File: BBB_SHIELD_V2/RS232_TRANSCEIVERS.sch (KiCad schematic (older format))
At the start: 13 parts, among them J4 Conn_02x05_Odd_Even

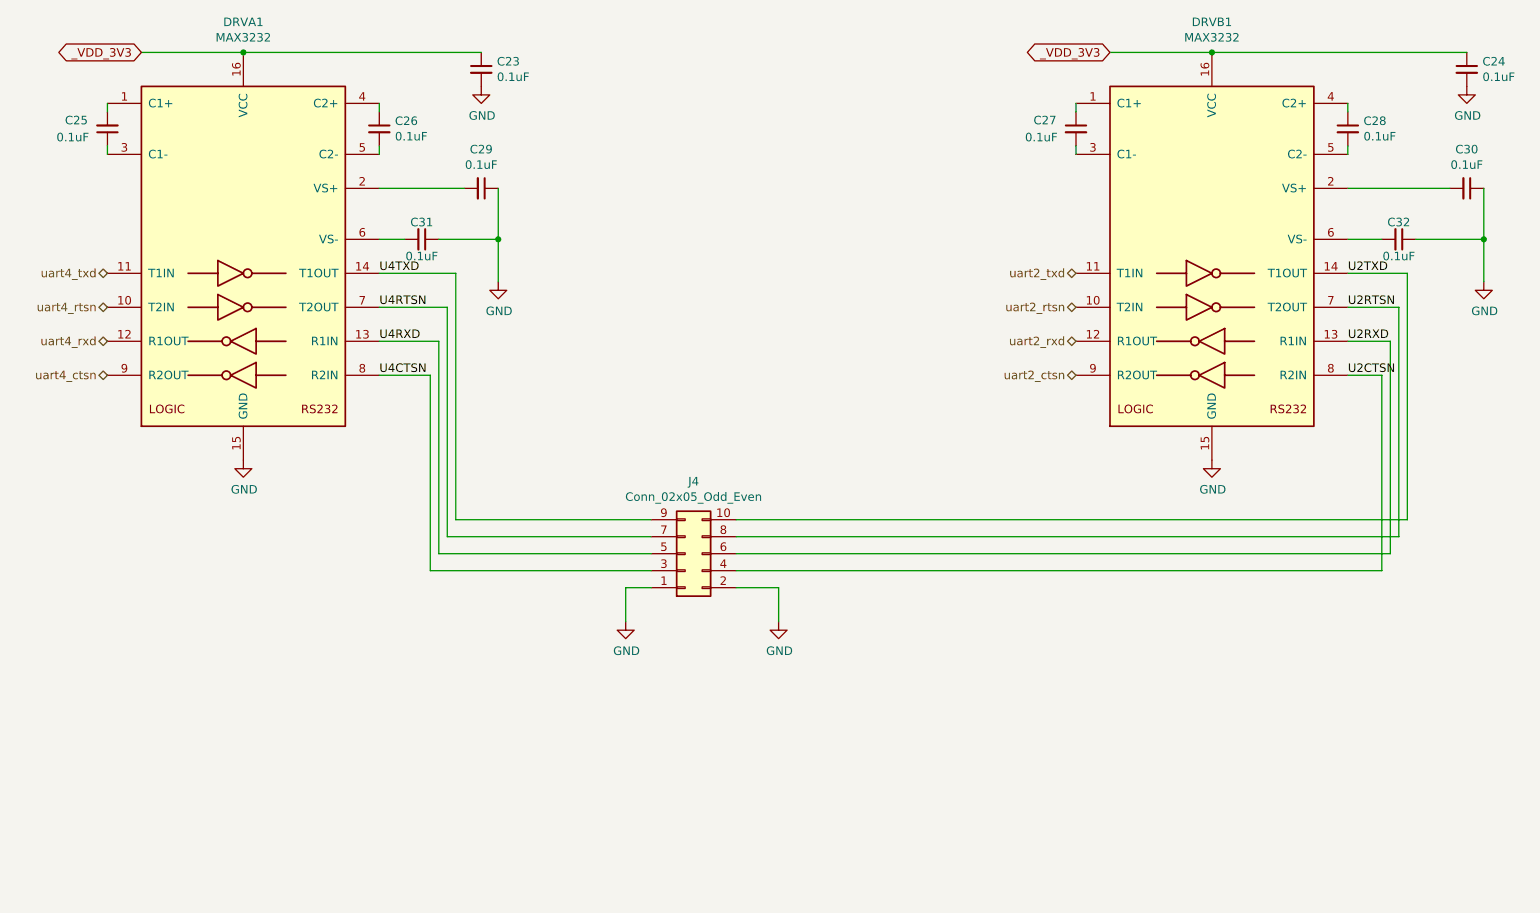
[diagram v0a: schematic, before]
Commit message: Schematic cleanup and refinement.
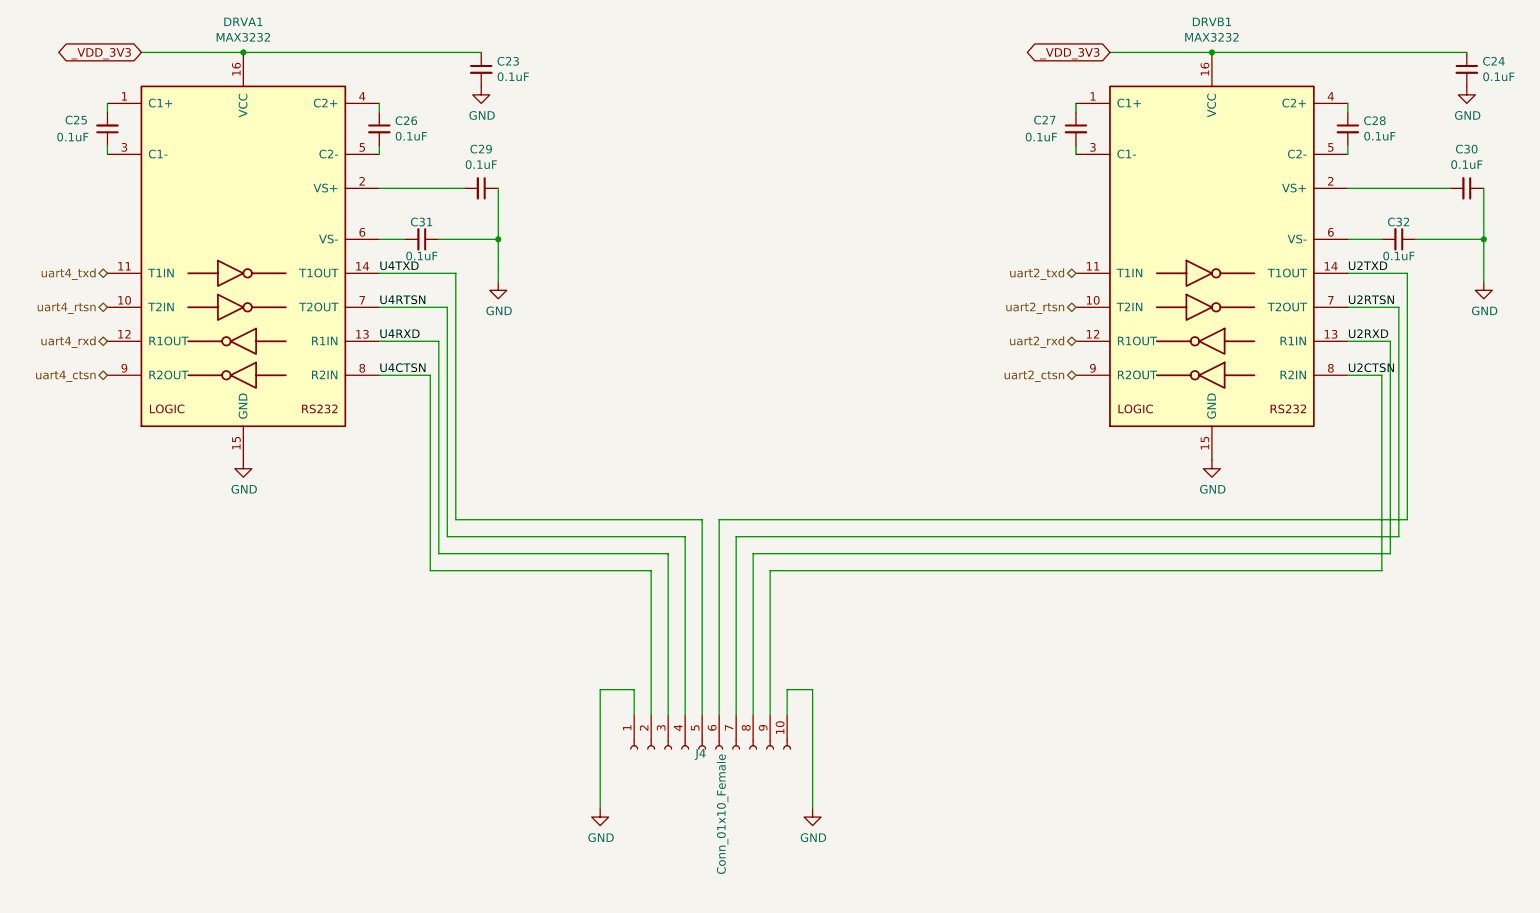
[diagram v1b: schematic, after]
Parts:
- removed J4: Conn_02x05_Odd_Even, CUSTOM_FOOTPRINTS:PCB TERMINAL BLOCK - 1841526, symbol Connector_Generic:Conn_02x05_Odd_Even
- added J4: Conn_01x10_Female, CUSTOM_FOOTPRINTS:10_POS_SPRING_TERM, symbol Connector:Conn_01x10_Female
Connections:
- net GND: now also J4.1 (Pin_1), J4.10 (Pin_10)
- net U2CTSN: now also J4.9 (Pin_9)
- net U2RTSN: now also J4.7 (Pin_7)
- net U2RXD: now also J4.8 (Pin_8)
- net U2TXD: now also J4.6 (Pin_6)
- net U4CTSN: now also J4.2 (Pin_2)
- net U4RTSN: now also J4.4 (Pin_4)
- net U4RXD: now also J4.3 (Pin_3)
- net U4TXD: now also J4.5 (Pin_5)
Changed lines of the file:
@@
 	1550 2600 2150 2600
 Connection ~ 2150 2600
-$Comp
-L Connector_Generic:Conn_02x05_Odd_Even J4
-U 1 1 5BF40240
-P 4750 5550
-F 0 "J4" H 4800 5125 50  0000 C CNN
-F 1 "Conn_02x05_Odd_Even" H 4800 5216 50  0000 C CNN
-F 2 "CUSTOM_FOOTPRINTS:PCB TERMINAL BLOCK - 1841526" H 4750 5550 50  0001 C CNN
-F 3 "" H 4750 5550 50  0001 C CNN
-F 4 "277-10318-ND" H 4750 5550 50  0001 C CNN "DKPN"
-F 5 "1841526" H 4750 5550 50  0001 C CNN "MFGPN"
-F 6 "BULK, VER 2018-12-09" H 0   0   50  0001 C CNN "NOTES"
-	1    4750 5550
-	1    0    0    1
-$EndComp
 Wire Wire Line
 	2950 3900 3400 3900
@@
 	3250 5650 4550 5650
 Wire Wire Line
-	3300 5550 4550 5550
-Wire Wire Line
-	3350 5450 4550 5450
-Wire Wire Line
-	3400 5350 4550 5350
-Wire Wire Line
 	8650 4100 8950 4100
 Wire Wire Line
@@
 	8900 4300 8900 5550
 Wire Wire Line
-	8900 5550 5050 5550
-Wire Wire Line
-	5050 5650 8850 5650
+	8900 5550 5150 5550
 Wire Wire Line
 	8850 5650 8850 4500
@@
 	8650 3900 9000 3900
 Wire Wire Line
-	5050 5350 9000 5350
-Wire Wire Line
 	9000 3900 9000 5350
-Wire Wire Line
-	4550 5750 4400 5750
-Wire Wire Line
-	4400 5750 4400 5950
-Wire Wire Line
-	5050 5750 5300 5750
-Wire Wire Line
-	5300 5750 5300 5950
 $Comp
 L power:GND #PWR054
 U 1 1 5BF49E20
-P 5300 5950
-F 0 "#PWR054" H 5300 5700 50  0001 C CNN
-F 1 "GND" H 5305 5777 50  0000 C CNN
-F 2 "" H 5300 5950 50  0001 C CNN
-F 3 "" H 5300 5950 50  0001 C CNN
-	1    5300 5950
+P 5500 7050
+F 0 "#PWR054" H 5500 6800 50  0001 C CNN
+F 1 "GND" H 5505 6877 50  0000 C CNN
+F 2 "" H 5500 7050 50  0001 C CNN
+F 3 "" H 5500 7050 50  0001 C CNN
+	1    5500 7050
 	1    0    0    -1
 $EndComp
@@
 L power:GND #PWR053
 U 1 1 5BF49E69
-P 4400 5950
-F 0 "#PWR053" H 4400 5700 50  0001 C CNN
-F 1 "GND" H 4405 5777 50  0000 C CNN
-F 2 "" H 4400 5950 50  0001 C CNN
-F 3 "" H 4400 5950 50  0001 C CNN
-	1    4400 5950
+P 4250 7050
+F 0 "#PWR053" H 4250 6800 50  0001 C CNN
+F 1 "GND" H 4255 6877 50  0000 C CNN
+F 2 "" H 4250 7050 50  0001 C CNN
+F 3 "" H 4250 7050 50  0001 C CNN
+	1    4250 7050
 	1    0    0    -1
 $EndComp
@@
 Text Label 2950 4500 0    50   ~ 0
 U4CTSN
+$Comp
+L Connector:Conn_01x10_Female J4
+U 1 1 5D15C1E2
+P 4850 6700
+F 0 "J4" V 4877 6676 50  0000 L CNN
+F 1 "Conn_01x10_Female" H 4877 6585 50  0000 L CNN
+F 2 "CUSTOM_FOOTPRINTS:10_POS_SPRING_TERM" H 4850 6700 50  0001 C CNN
+F 3 "~" H 4850 6700 50  0001 C CNN
+	1    4850 6700
+	0    -1   1    0
+$EndComp
+Wire Wire Line
+	4250 6350 4450 6350
+Wire Wire Line
+	4450 6350 4450 6500
+Wire Wire Line
+	4250 6350 4250 7050
+Wire Wire Line
+	5350 6500 5350 6350
+Wire Wire Line
+	5350 6350 5500 6350
+Wire Wire Line
+	5500 6350 5500 7050
+Wire Wire Line
+	4550 5650 4550 6500
+Wire Wire Line
+	4650 5550 4650 6500
+Wire Wire Line
+	3300 5550 4650 5550
+Wire Wire Line
+	4750 5450 4750 6500
+Wire Wire Line
+	3350 5450 4750 5450
+Wire Wire Line
+	4850 5350 4850 6500
+Wire Wire Line
+	3400 5350 4850 5350
+Wire Wire Line
+	5250 5650 8850 5650
+Wire Wire Line
+	5250 6500 5250 5650
+Wire Wire Line
+	5150 5550 5150 6500
+Wire Wire Line
+	5050 6500 5050 5450
+Wire Wire Line
+	4950 5350 4950 6500
+Wire Wire Line
+	4950 5350 9000 5350
 $EndSCHEMATC

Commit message: Rev 2 problem fixes.
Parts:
- C23, C24, C25, C26, C27, C28, C29, C30, C31, C32: NOTES REEL, VER 2018-11-25 -> VER,2019-07-17,REEL
- DRVA1, DRVB1: NOTES BULK, VER 2018-11-25 -> VER,2019-07-15,CT
- J4: NOTES (none) -> VER,2019-07-16,BULK
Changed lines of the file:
@@
 F 4 "296-19851-1-ND" H 0   0   50  0001 C CNN "DKPN"
 F 5 "MAX3232ECDR" H 0   0   50  0001 C CNN "MFGPN"
-F 6 "BULK, VER 2018-11-25" H 0   0   50  0001 C CNN "NOTES"
+F 6 "VER,2019-07-15,CT" H 0   0   50  0001 C CNN "NOTES"
 	1    2150 3800
 	1    0    0    -1
@@
 F 4 "296-19851-1-ND" H 0   0   50  0001 C CNN "DKPN"
 F 5 "MAX3232ECDR" H 0   0   50  0001 C CNN "MFGPN"
-F 6 "BULK, VER 2018-11-25" H 0   0   50  0001 C CNN "NOTES"
+F 6 "VER,2019-07-15,CT" H 0   0   50  0001 C CNN "NOTES"
 	1    7850 3800
 	1    0    0    -1
@@
 F 7 "X7R" H 0   0   50  0001 C CNN "TEMPCO"
 F 8 "50" H 0   0   50  0001 C CNN "VOLTAGE"
-F 9 "REEL, VER 2018-11-25" H 0   0   50  0001 C CNN "NOTES"
+F 9 "VER,2019-07-17,REEL" H 0   0   50  0001 C CNN "NOTES"
 	1    1350 3050
 	-1   0    0    1
@@
 F 7 "X7R" H 0   0   50  0001 C CNN "TEMPCO"
 F 8 "50" H 0   0   50  0001 C CNN "VOLTAGE"
-F 9 "REEL, VER 2018-11-25" H 0   0   50  0001 C CNN "NOTES"
+F 9 "VER,2019-07-17,REEL" H 0   0   50  0001 C CNN "NOTES"
 	1    2950 3050
 	1    0    0    -1
@@
 F 7 "X7R" H 0   0   50  0001 C CNN "TEMPCO"
 F 8 "50" H 0   0   50  0001 C CNN "VOLTAGE"
-F 9 "REEL, VER 2018-11-25" H 0   0   50  0001 C CNN "NOTES"
+F 9 "VER,2019-07-17,REEL" H 0   0   50  0001 C CNN "NOTES"
 	1    3550 2700
 	1    0    0    -1
@@
 F 7 "X7R" H 0   0   50  0001 C CNN "TEMPCO"
 F 8 "50" H 0   0   50  0001 C CNN "VOLTAGE"
-F 9 "REEL, VER 2018-11-25" H 9350 2700 50  0001 C CNN "NOTES"
+F 9 "VER,2019-07-17,REEL" H 9350 2700 50  0001 C CNN "NOTES"
 	1    9350 2700
 	1    0    0    -1
@@
 F 7 "X7R" H 0   0   50  0001 C CNN "TEMPCO"
 F 8 "50" H 0   0   50  0001 C CNN "VOLTAGE"
-F 9 "REEL, VER 2018-11-25" H 0   0   50  0001 C CNN "NOTES"
+F 9 "VER,2019-07-17,REEL" H 0   0   50  0001 C CNN "NOTES"
 	1    3550 3400
 	0    1    1    0
@@
 F 7 "X7R" H 0   0   50  0001 C CNN "TEMPCO"
 F 8 "50" H 0   0   50  0001 C CNN "VOLTAGE"
-F 9 "REEL, VER 2018-11-25" H 0   0   50  0001 C CNN "NOTES"
+F 9 "VER,2019-07-17,REEL" H 0   0   50  0001 C CNN "NOTES"
 	1    3200 3700
 	0    1    1    0
@@
 F 7 "X7R" H 0   0   50  0001 C CNN "TEMPCO"
 F 8 "50" H 0   0   50  0001 C CNN "VOLTAGE"
-F 9 "REEL, VER 2018-11-25" H 0   0   50  0001 C CNN "NOTES"
+F 9 "VER,2019-07-17,REEL" H 0   0   50  0001 C CNN "NOTES"
 	1    7050 3050
 	1    0    0    -1
@@
 F 7 "X7R" H 0   0   50  0001 C CNN "TEMPCO"
 F 8 "50" H 0   0   50  0001 C CNN "VOLTAGE"
-F 9 "REEL, VER 2018-11-25" H 0   0   50  0001 C CNN "NOTES"
+F 9 "VER,2019-07-17,REEL" H 0   0   50  0001 C CNN "NOTES"
 	1    8650 3050
 	1    0    0    -1
@@
 F 7 "X7R" H 0   0   50  0001 C CNN "TEMPCO"
 F 8 "50" H 0   0   50  0001 C CNN "VOLTAGE"
-F 9 "REEL, VER 2018-11-25" H 0   0   50  0001 C CNN "NOTES"
+F 9 "VER,2019-07-17,REEL" H 0   0   50  0001 C CNN "NOTES"
 	1    9350 3400
 	0    1    1    0
@@
 F 7 "X7R" H 0   0   50  0001 C CNN "TEMPCO"
 F 8 "50" H 0   0   50  0001 C CNN "VOLTAGE"
-F 9 "REEL, VER 2018-11-25" H 0   0   50  0001 C CNN "NOTES"
+F 9 "VER,2019-07-17,REEL" H 0   0   50  0001 C CNN "NOTES"
 	1    8950 3700
 	0    1    1    0
@@
 F 2 "CUSTOM_FOOTPRINTS:10_POS_SPRING_TERM" H 4850 6700 50  0001 C CNN
 F 3 "~" H 4850 6700 50  0001 C CNN
+F 4 "VER,2019-07-16,BULK" H 0   0   50  0001 C CNN "NOTES"
 	1    4850 6700
 	0    -1   1    0
